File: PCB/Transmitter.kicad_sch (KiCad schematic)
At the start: 31 parts, among them T1 MABA-007159, U1 LTC5599IUF, U2 ADF4351

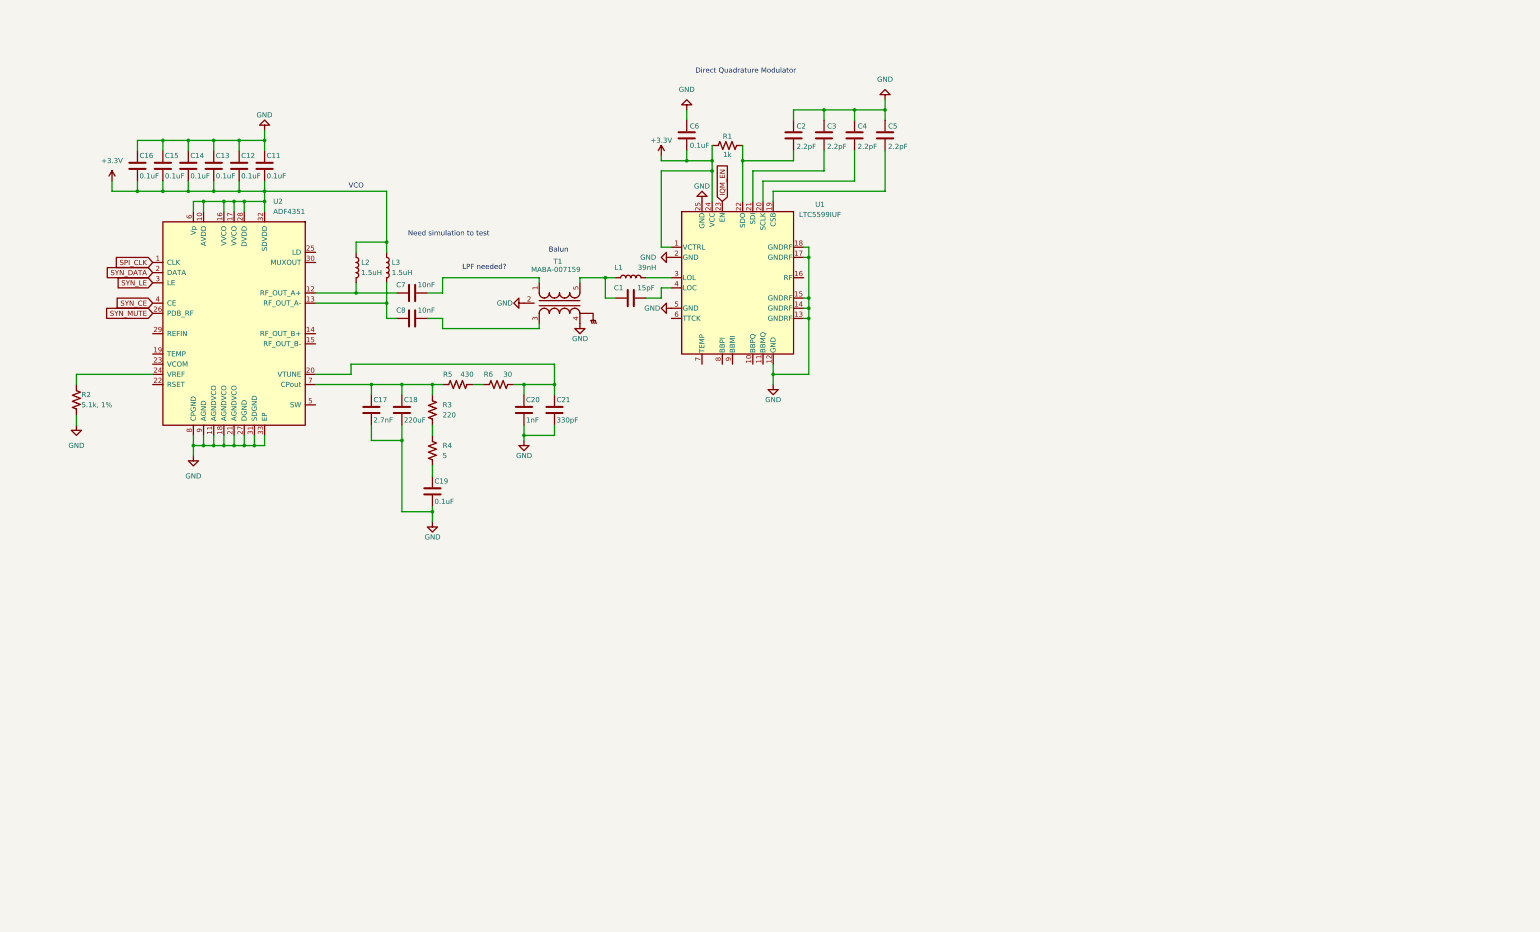
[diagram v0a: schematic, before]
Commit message: new file:   Datasheet/HMC849A_RF_Switch_SPDT.pdf 	new file:   Datasheet/TG2016SMN_26MHz_MCGNNM_Oscillator.pdf 	modified:   PCB/DroidRadio.kicad_pro 	modified:   PCB/DroidRadio.kicad_sch 	modified:   PCB/Processors.kicad_sch 	modified:   PCB/Simulation/Transmitter_Side.pll 	modified:   PCB/Transmitter.kicad_sch 	deleted:    PCB/~DroidRadio.kicad_pro.lck
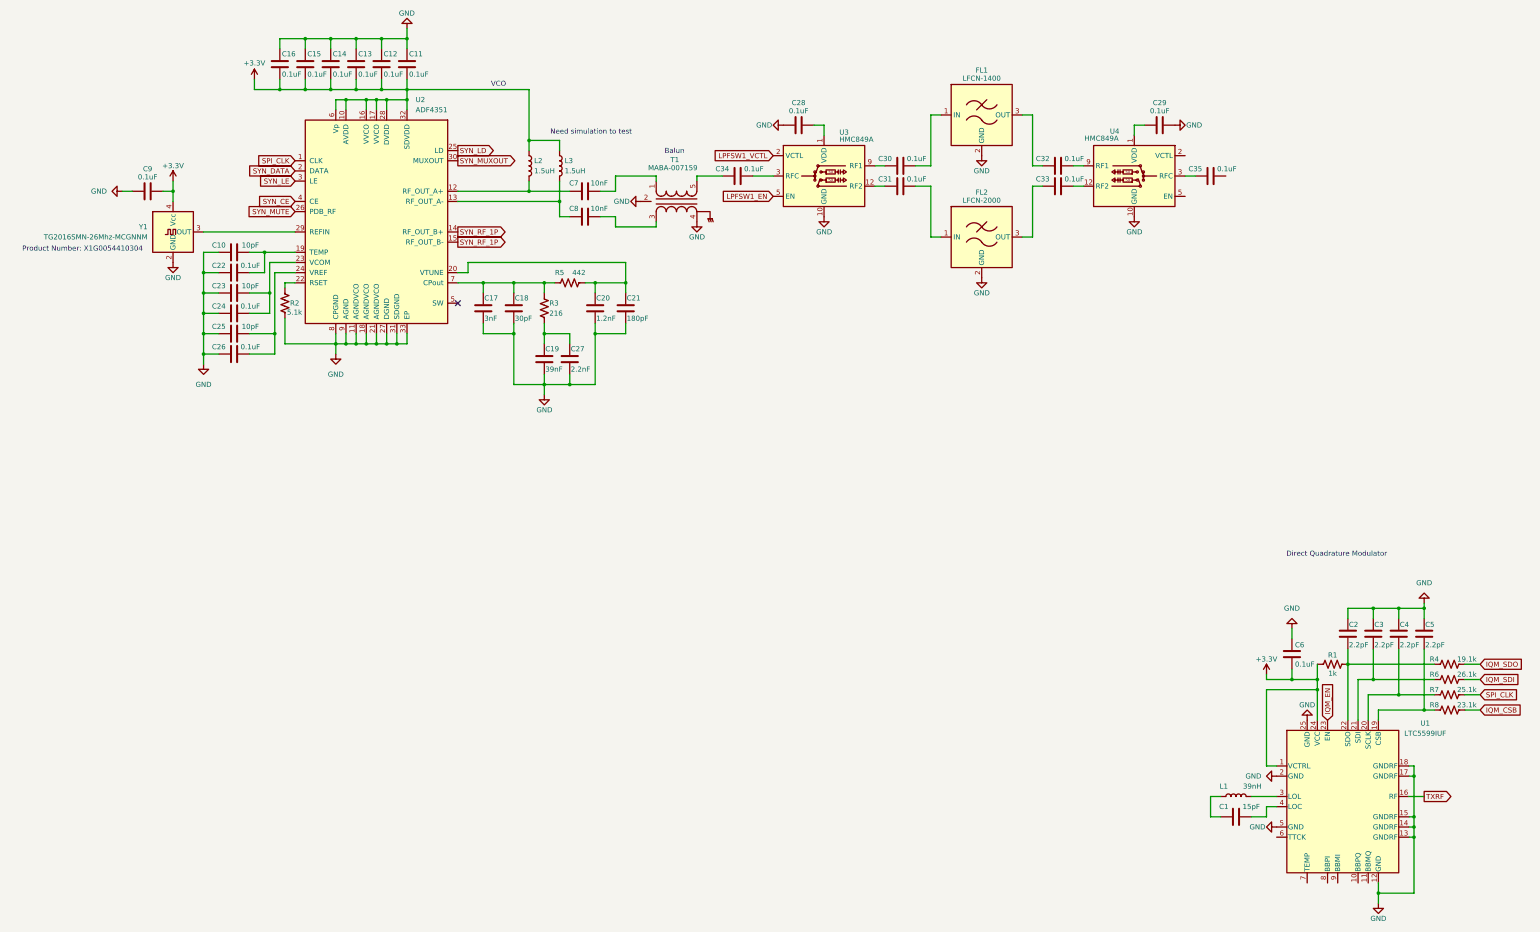
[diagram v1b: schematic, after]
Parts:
- added C10, C23, C25: 10pF, symbol Device:C
- added C22, C24, C26, C28, C29, C30, C31, C32, C33, C34, C35, C9: 0.1uF, symbol Device:C
- added C27: 2.2nF, symbol Device:C
- added FL1: LFCN-1400, Filter:Filter_Mini-Circuits_FV1206, symbol RF_Filter:LFCN-1400
- added FL2: LFCN-2000, Filter:Filter_Mini-Circuits_FV1206, symbol RF_Filter:LFCN-2000
- added R7: 25.1k, symbol Device:R_US
- added R8: 23.1k, symbol Device:R_US
- added U3, U4: HMC849A, Package_DFN_QFN:QFN-24-1EP_4x4mm_P0.5mm_EP2.65x2.65mm_ThermalVias, symbol RF_Switch:HMC849A
- added Y1: TG2016SMN-26Mhz-MCGNNM, Crystal:Crystal_SMD_2016-4Pin_2.0x1.6mm, symbol Oscillator:TG2520SMN-xx.xxxxxxMhz-xxxxNM
- C17: value 2.7nF -> 3nF; Tolerance (none) -> 1%
- C18: value 220uF -> 30pF; Tolerance (none) -> 1%
- C19: value 0.1uF -> 39nF; Tolerance (none) -> 1%
- C20: value 1nF -> 1.2nF; Tolerance (none) -> 1%
- C21: value 330pF -> 180pF; Tolerance (none) -> 1%
- R2: value 5.1k, 1% -> 5.1k; Tolerance (none) -> 1%
- R3: value 220 -> 216; Tolerance (none) -> 1%
- R4: value 5 -> 19.1k
- R5: value 430 -> 442; Tolerance (none) -> 1%
- R6: value 30 -> 26.1k
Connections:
- net +3.3V: now also C9.2, Y1.4 (Vcc)
- net GND: now also C10.1, C22.1, C23.1, C24.1, C25.1, C26.1, C27.2, C28.1, C29.2, C9.1, FL1.2 (GND), FL1.4 (GND), FL2.2 (GND), FL2.4 (GND), U3.10 (GND), U3.11 (GND), U3.13 (GND), U3.14 (GND), U3.15 (GND), U3.16 (GND), U3.17 (GND), U3.4 (GND), U3.6 (GND), U3.7 (GND), U3.8 (GND), U4.10 (GND), U4.11 (GND), U4.13 (GND), U4.14 (GND), U4.15 (GND), U4.16 (GND), U4.17 (GND), U4.4 (GND), U4.6 (GND), U4.7 (GND), U4.8 (GND), Y1.2 (GND)
- net SPI_CLK: now also R7.2
- net at C1.1, L1.1: no longer T1.5
- net at C19.1: now also R3.2, C27.1; no longer R4.2
- net at C20.1, C21.1, U2.20 (VTUNE): now also R5.2; no longer R6.2
- net at C5.2, U1.19 (CSB): now also R8.1
- net at R6.1: now also C3.2, U1.21 (SDI); no longer R5.2
- net at C4.2, U1.20 (SCLK): now also R7.1
- net at R2.1: now also U2.22 (RSET); no longer U2.24 (VREF)
- net at R4.1: now also C2.2, R1.2, U1.22 (SDO); no longer R3.2
- net TXRF: now reaches U1.16 (RF)
- net SYN_RF_1P: now reaches U2.14 (RF_OUT_B+)
- net SYN_RF_1P: now also U2.15 (RF_OUT_B-)
- net at U2.19 (TEMP): now also C10.2, C22.2
- net at U2.23 (VCOM): now also C23.2, C24.2
- net SYN_LD: now reaches U2.25 (LD)
- net at U2.29 (REFIN): now also Y1.3 (OUT)
- net SYN_MUXOUT: now reaches U2.30 (MUXOUT)
- new net: C33.1, FL2.3 (OUT)
- new net: C33.2, U4.12 (RF2)
- new net: C31.1, U3.12 (RF2)
- new net: C31.2, FL2.1 (IN)
- new net: C35.1, U4.3 (RFC)
- new net: C29.1, U4.1 (VDD)
- new net: C32.2, U4.9 (RF1)
- new net: C34.1, T1.5
- new net: C34.2, U3.3 (RFC)
- new net: C30.1, U3.9 (RF1)
- new net: C30.2, FL1.1 (IN)
- new net: C28.2, U3.1 (VDD)
- new net: C25.2, C26.2, U2.24 (VREF)
- new net: C32.1, FL1.3 (OUT)
- new net IQM_CSB: R8.2
- new net IQM_SDI: R6.2
- new net IQM_SDO: R4.2
- new net LPFSW1_EN: U3.5 (EN)
- new net LPFSW1_VCTL: U3.2 (VCTL)
- no-connect marks 0 -> 1
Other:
- note added: "Product Number: X1G0054410304"
- note removed: "LPF needed?"
- moved on the sheet: C1, C11, C12, C13, C14, C15, C16, C17, C18, C2, C20, C21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
